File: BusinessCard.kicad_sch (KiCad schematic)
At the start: 64 parts, among them J1 RST, J3 USB_C_Receptacle_USB2.0_14P, SW1 SW_Push, SW10 SW_Push, SW11 SW_Push, SW12 SW_Push, SW13 SW_Push, SW14 SW_Push, SW15 SW_Push, SW16 SW_Push, SW2 SW_Push, SW3 SW_Push, SW4 SW_Push, SW5 SW_Push, SW6 SW_Push, SW7 SW_Push, SW8 SW_Push, SW9 SW_Push, U2 USBLC6-2SC6, U3 ATmega32U4-M, Y1 X322516MLB4SI

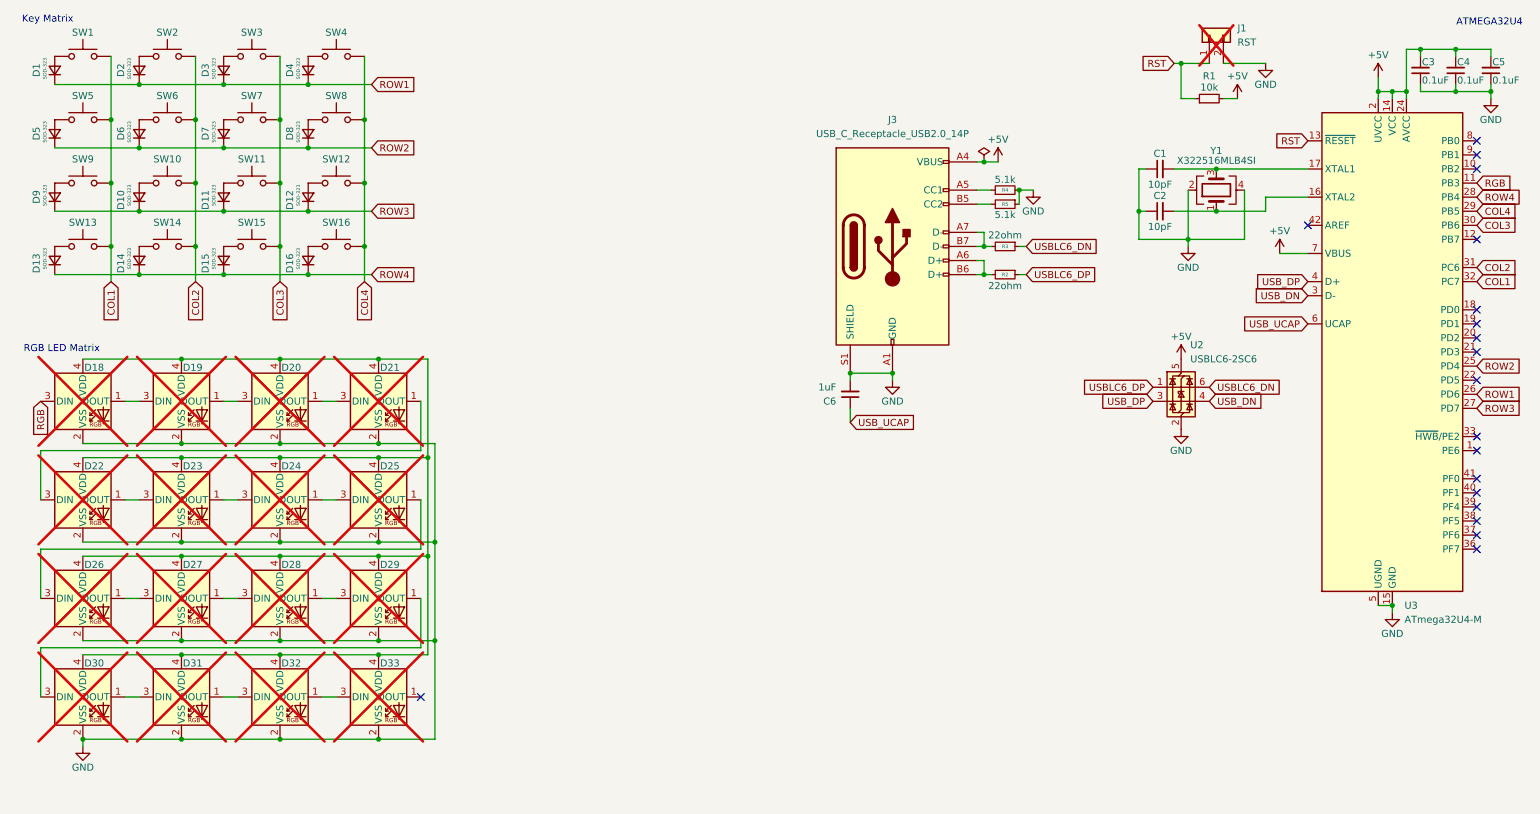
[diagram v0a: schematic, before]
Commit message: Update
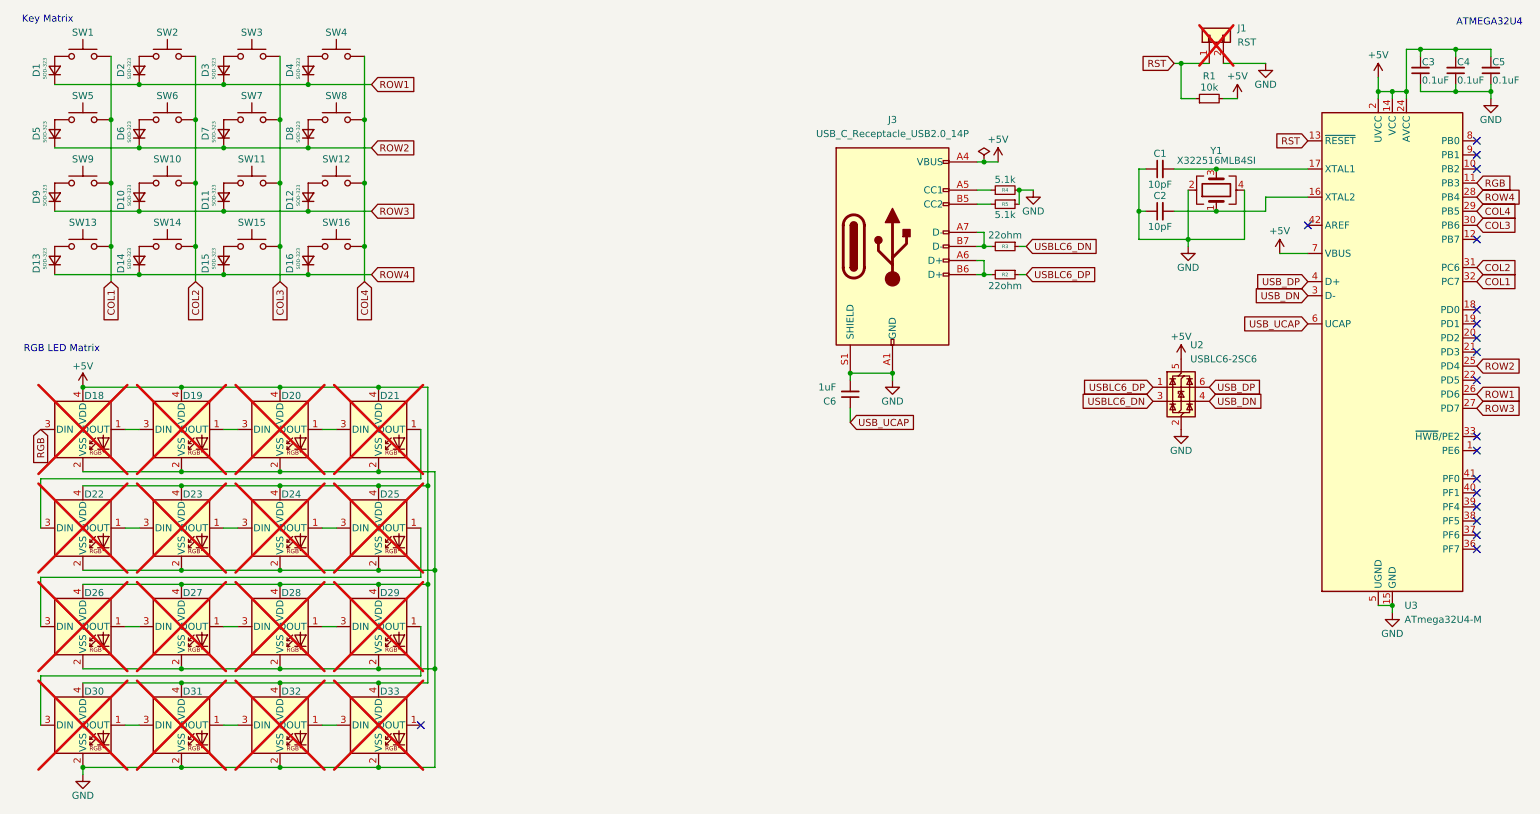
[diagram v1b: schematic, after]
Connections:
- net +5V: now also D18.4 (VDD), D19.4 (VDD), D20.4 (VDD), D21.4 (VDD), D22.4 (VDD), D23.4 (VDD), D24.4 (VDD), D25.4 (VDD), D26.4 (VDD), D27.4 (VDD), D28.4 (VDD), D29.4 (VDD), D30.4 (VDD), D31.4 (VDD), D32.4 (VDD), D33.4 (VDD)
- net USBLC6_DN: now also U2.3 (I/O2); no longer U2.6 (I/O1)
- net USB_DP: now also U2.6 (I/O1); no longer U2.3 (I/O2)
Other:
- moved on the sheet: D18, D19, D20, D21, D22, D23, D24, D25, D26, D27, D28, D29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
